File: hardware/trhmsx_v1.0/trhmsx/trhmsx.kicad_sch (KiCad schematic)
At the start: 52 parts, among them J1 Micro_SD_Card_Det1, J2 Mini-DIN-6, J3 USB_A, J4 Barrel_Jack, J5 Conn_01x02, J6 Conn_01x05, J7 Conn_02x25_Odd_Even, J8 Conn_02x25_Odd_Even, SW1 SW_Push, SW2 SW_DIP_x08, U1 EP1C12Q240C8N, U2 AMS1117-1.5, U3 AMS1117-3.3, U4 M51953BFP, U5 NC7WZU04P6X, Y1 Crystal

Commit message: working on the base circuit
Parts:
- removed J2: Mini-DIN-6, symbol Connector:Mini-DIN-6
- removed J3: USB_A, symbol Connector:USB_A
- removed R3, R4: 1K, symbol Device:R
- added C13, C14, C15, C16, C17, C18, C19, C20: 220uF, symbol Device:C_Polarized
- added J12: USB_A_Stacked, symbol Connector:USB_A_Stacked
- added J13: Mini-DIN-6, symbol Connector:Mini-DIN-6
- added J2: RCA, symbol Connector:Conn_Coaxial
- added J3: DH15, symbol Connector:DA15_Receptacle
- added J9: AudioJack2_Ground, symbol Connector_Audio:AudioJack2_Ground
- added R11, R12, R8: 1K, symbol Device:R
- added R13, R14: 330, symbol Device:R
- added RN10, RN12, RN14, RN16, RN18, RN20, RN22, RN8: 200, symbol Device:R_Pack04_Split
- added RN11, RN13, RN15, RN17, RN19, RN21, RN23, RN9: 100, symbol Device:R_Pack04_Split
- added U6: 4053, symbol 4xxx:4053
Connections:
- net +3.3V: now also R11.1, R12.1
- net +5V: now also J12.1 (VBUS1), J12.5 (VBUS2), J13.4, J3.9 (P9)
- net GND: now also J12.4 (GND1), J12.8 (GND2), J12.9 (Shield), J13.3, J2.2 (Ext), J3.10 (P10), J3.5, J3.6, J3.7, J3.8, J9.G, RN11.2 (R2.1), RN13.4 (R4.1), RN17.2 (R2.1), RN19.4 (R4.1), RN23.2 (R2.1)
- net KCLK: now also J12.3 (D1+), J13.5, R11.2
- net KDAT: now also J12.2 (D1-), J13.1, R12.2
- net PWRLED: now also R8.1; no longer D9.2 (A)
- net SOUND_L: now also C14.2, J9.T
- new net: RN14.3 (R3.1), RN15.2 (R2.1), RN15.6 (R3.2)
- new net: RN14.2 (R2.1), RN15.1 (R1.1), RN15.7 (R2.2)
- new net: RN20.2 (R2.1), RN21.1 (R1.1), RN21.7 (R2.2)
- new net: RN12.2 (R2.1), RN13.1 (R1.1), RN13.7 (R2.2)
- new net: RN11.4 (R4.1), RN12.1 (R1.1), RN13.8 (R1.2)
- new net: RN16.2 (R2.1), RN17.1 (R1.1), RN17.7 (R2.2)
- new net: RN15.4 (R4.1), RN16.1 (R1.1), RN17.8 (R1.2)
- new net: RN18.4 (R4.1), RN19.3 (R3.1), RN19.5 (R4.2)
- new net: C14.1, RN10.3 (R3.1), RN11.6 (R3.2)
- new net: RN17.4 (R4.1), RN18.1 (R1.1), RN19.8 (R1.2)
- new net: RN12.4 (R4.1), RN13.3 (R3.1), RN13.5 (R4.2)
- new net: C13.1, RN8.1 (R1.1), RN9.8 (R1.2)
- new net: RN14.4 (R4.1), RN15.3 (R3.1), RN15.5 (R4.2)
- new net: RN10.1 (R1.1), RN11.8 (R1.2), RN9.4 (R4.1)
- new net: C18.2, J3.1
- new net: C19.2, J3.2
- new net: C20.2, J3.3
- new net: RN20.4 (R4.1), RN21.3 (R3.1), RN21.5 (R4.2)
- new net: RN20.3 (R3.1), RN21.2 (R2.1), RN21.6 (R3.2)
- new net: RN18.3 (R3.1), RN19.2 (R2.1), RN19.6 (R3.2)
- new net: RN10.4 (R4.1), RN11.3 (R3.1), RN11.5 (R4.2)
- new net: RN21.4 (R4.1), RN22.1 (R1.1), RN23.8 (R1.2)
- new net: RN10.2 (R2.1), RN11.1 (R1.1), RN11.7 (R2.2)
- new net: RN8.2 (R2.1), RN9.1 (R1.1), RN9.7 (R2.2)
- new net: D9.2 (A), R8.2
- new net: RN8.4 (R4.1), RN9.3 (R3.1), RN9.5 (R4.2)
- new net: RN22.2 (R2.1), RN23.1 (R1.1), RN23.7 (R2.2)
- new net: RN12.3 (R3.1), RN13.2 (R2.1), RN13.6 (R3.2)
- new net: RN8.3 (R3.1), RN9.2 (R2.1), RN9.6 (R3.2)
- new net: RN18.2 (R2.1), RN19.1 (R1.1), RN19.7 (R2.2)
- new net: RN16.4 (R4.1), RN17.3 (R3.1), RN17.5 (R4.2)
- new net: J12.6 (D2-), R14.2
- new net: J12.7 (D2+), R13.1
- new net HSYNC: J3.13 (P13)
- new net SCLK: J3.12 (P12)
- new net SDAT: J3.15 (P15)
- new net SL0: RN12.5 (R4.2)
- new net SL1: RN12.6 (R3.2)
- new net SL2: RN12.7 (R2.2)
- new net SL3: RN12.8 (R1.2)
- new net SL4: RN10.5 (R4.2)
- new net SL5: RN10.6 (R3.2)
- new net SOUND_R: C13.2, J9.S
- new net SR0: RN10.7 (R2.2)
- new net SR1: RN10.8 (R1.2)
- new net SR2: RN8.5 (R4.2)
- new net SR3: RN8.6 (R3.2)
- new net SR4: RN8.7 (R2.2)
- new net SR5: RN8.8 (R1.2)
- new net USBN1: R13.2
- new net USBP1: R14.1
- new net VB0: RN16.7 (R2.2)
- new net VB1: RN16.8 (R1.2)
- new net VB2: RN14.5 (R4.2)
- new net VB3: RN14.6 (R3.2)
- new net VB4: RN14.7 (R2.2)
- new net VB5: RN14.8 (R1.2)
- new net VBO: C15.1, RN14.1 (R1.1), RN15.8 (R1.2)
- new net VBX: C20.1, U6.4 (Z)
- new net VB_CV: C15.2, J2.1 (In)
- new net VG0: RN18.5 (R4.2)
- new net VG1: RN18.6 (R3.2)
- new net VG2: RN18.7 (R2.2)
- new net VG3: RN18.8 (R1.2)
- new net VG4: RN16.5 (R4.2)
- new net VG5: RN16.6 (R3.2)
- new net VGO: C16.1, RN16.3 (R3.1), RN17.6 (R3.2)
- new net VGX: C19.1, U6.15 (Y)
- new net VG_SY: C16.2
- new net VR0: RN22.7 (R2.2)
- new net VR1: RN22.8 (R1.2)
- new net VR2: RN20.5 (R4.2)
- new net VR3: RN20.6 (R3.2)
- new net VR4: RN20.7 (R2.2)
- new net VR5: RN20.8 (R1.2)
- new net VRO: C17.1, RN20.1 (R1.1), RN21.8 (R1.2)
- new net VRX: C18.1, U6.14 (X)
- new net VR_SC: C17.2
- new net VSYNC: J3.14 (P14)
- no-connect marks 3 -> 13
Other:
- moved on the sheet: D1, D2, D3, D4, D5, D6, D7, D8, D9, SW2

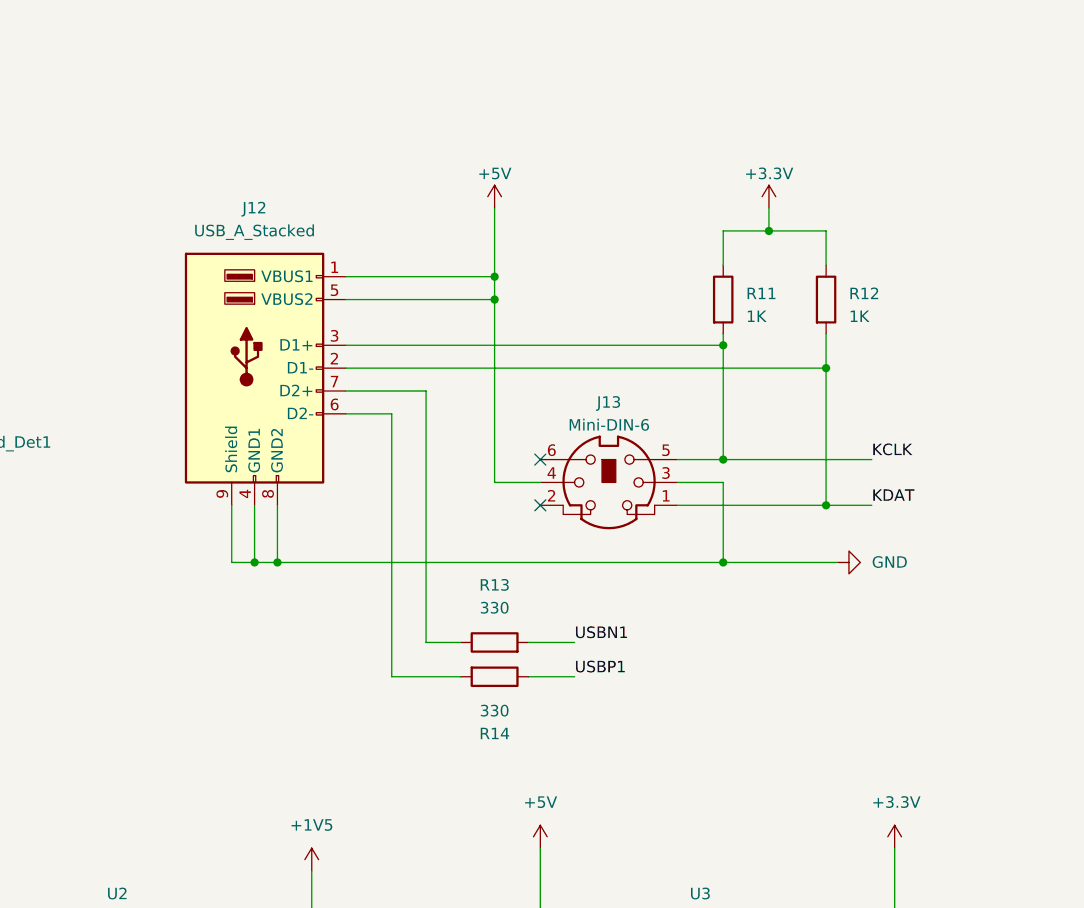
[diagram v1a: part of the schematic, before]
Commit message: USB-PS2
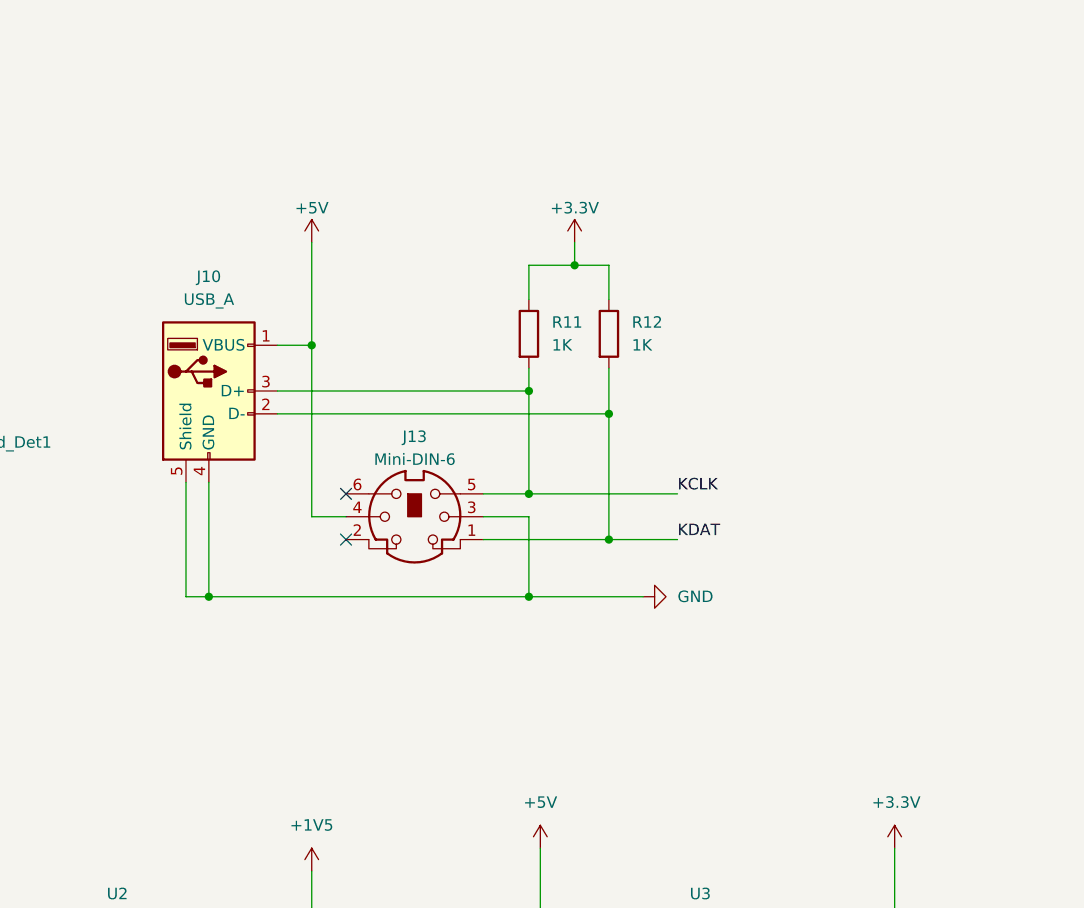
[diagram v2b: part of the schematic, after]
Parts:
- removed J12: USB_A_Stacked, symbol Connector:USB_A_Stacked
- removed R13, R14: 330, symbol Device:R
- added J10: USB_A, symbol Connector:USB_A
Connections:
- net +5V: now also J10.1 (VBUS)
- net GND: now also J10.4 (GND), J10.5 (Shield)
- net KCLK: now also J10.3 (D+)
- net KDAT: now also J10.2 (D-)
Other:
- moved on the sheet: J13, R11, R12
